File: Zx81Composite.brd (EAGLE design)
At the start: 24 x 42 mm, 14 parts, among them IC1 555, Q1 BC548, T1 2N2222

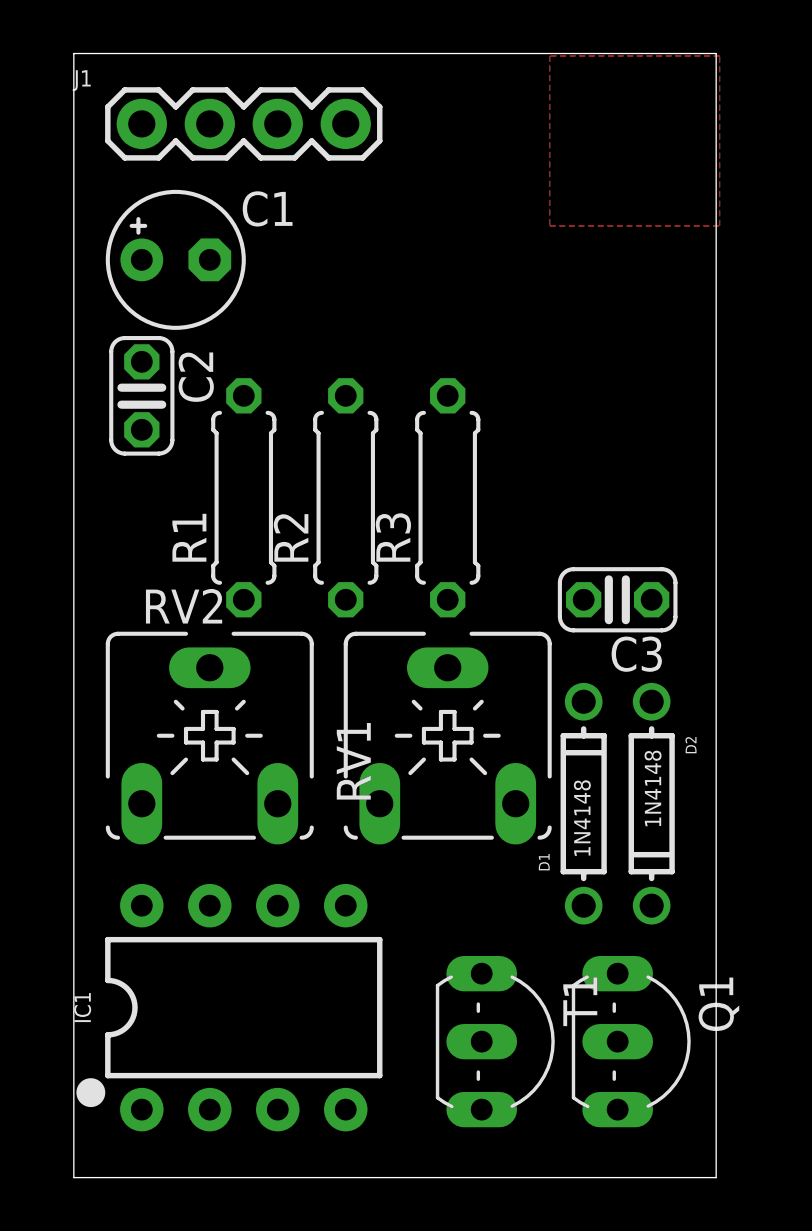
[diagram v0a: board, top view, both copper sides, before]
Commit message: Change implementation
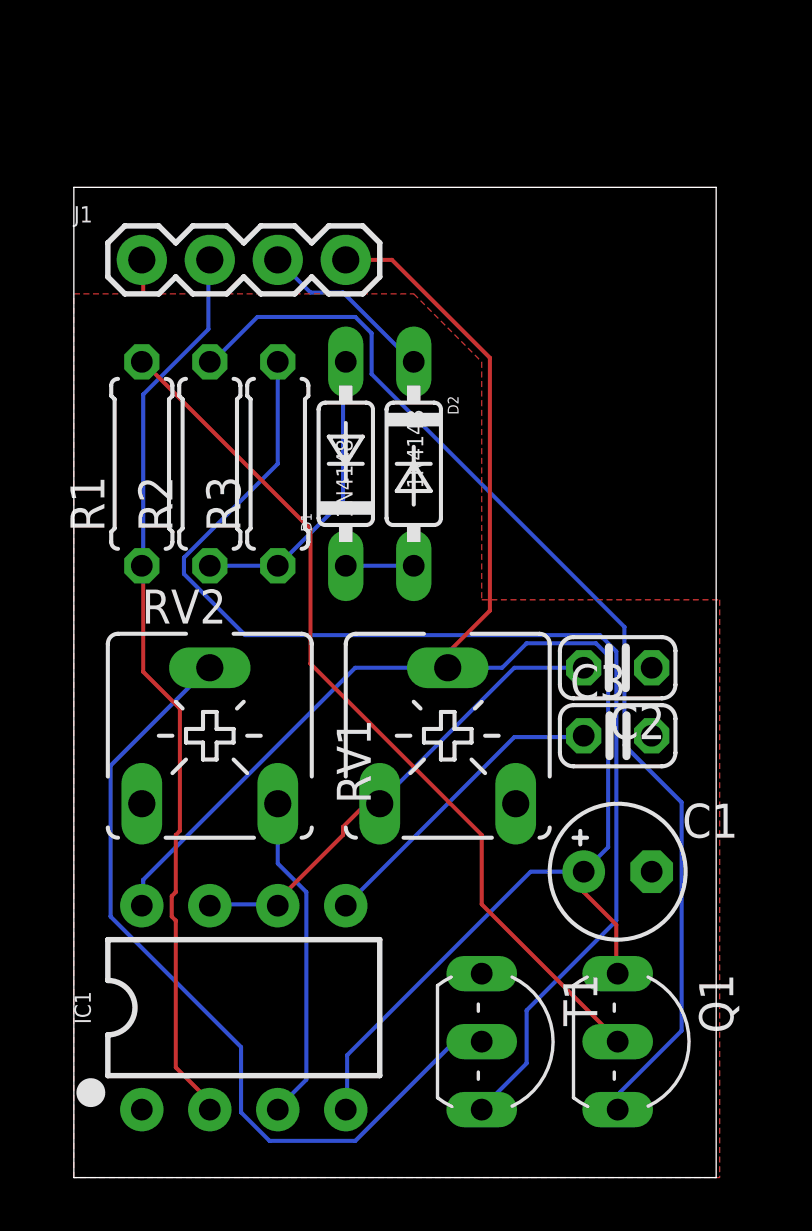
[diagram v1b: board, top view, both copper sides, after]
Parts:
- D1, D2: device adafruit:DO-1N4148 -> diode:DO35-7
- R2: value 56 -> 91
- moved C1 28.2 mm to (20.3, 11.4)
- moved C2 20.5 mm to (20.3, 19.1), turned to 180 degrees
- moved D1 15.5 mm to (10.2, 26.7)
- moved D2 15.5 mm to (12.7, 26.7)
- moved R3 6.48 mm to (7.62, 26.7)
- moved R2 5.24 mm to (5.08, 26.7)
- moved C3 5.08 mm to (20.3, 16.5), turned to 0 degrees
- moved J1 5.08 mm to (2.54, 34.3)
- moved R1 4.02 mm to (2.54, 26.7)
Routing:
- net VCC: track 0.00 -> 67.9 mm
- net N$8: track 0.00 -> 45.9 mm
- net N$11: track 0.00 -> 41.8 mm
- net ULA: track 0.00 -> 34.2 mm
- net N$1: track 0.00 -> 32.8 mm
- net N$3: track 0.00 -> 31.2 mm
- net N$5: track 0.00 -> 18.1 mm
- net N$6: track 0.00 -> 12.3 mm
- net N$4: track 0.00 -> 11.6 mm
- net N$7: track 0.00 -> 11.3 mm
- net AVOUT: track 0.00 -> 6.66 mm
- net N$2: track 0.00 -> 2.54 mm
- net GND: track 0.00 -> 1.32 mm
- added copper zone on layer 1, net GND
- removed copper zone on layer 1, net N$9
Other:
- board size 24 x 42 mm -> 24 x 37 mm
